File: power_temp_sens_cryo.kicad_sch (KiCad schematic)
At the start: 20 parts, among them J1 temp. sens., J2 MCU_ADC1, J3 MCU_ADC0, J4 5V, J5 GND, U1 AD8276, U2 AD8603, U3 AD8276, U4 AD8603

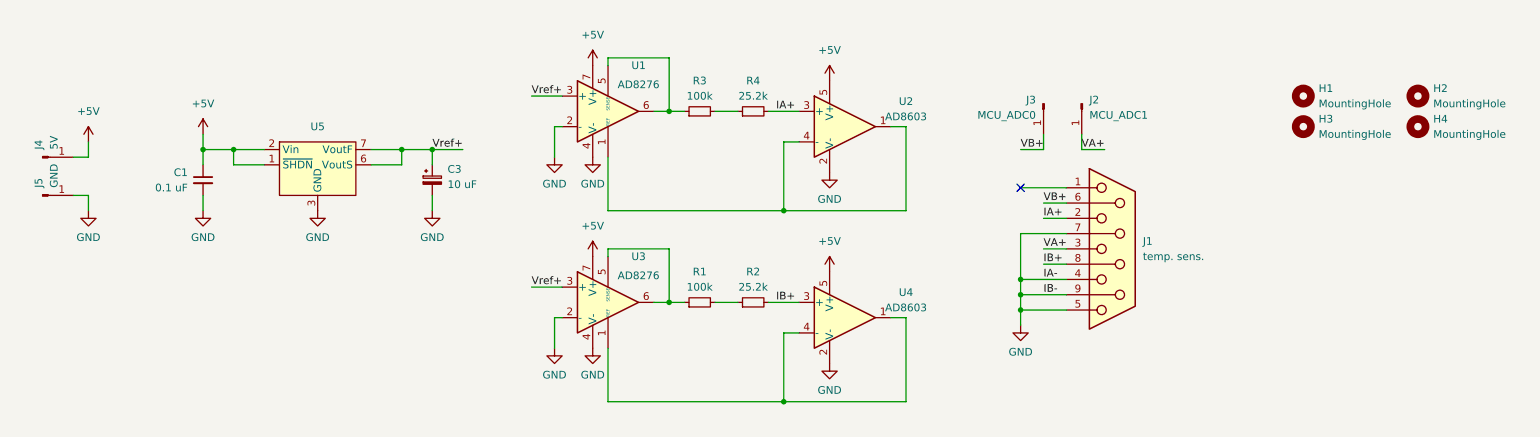
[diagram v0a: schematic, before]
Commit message: unfinished project
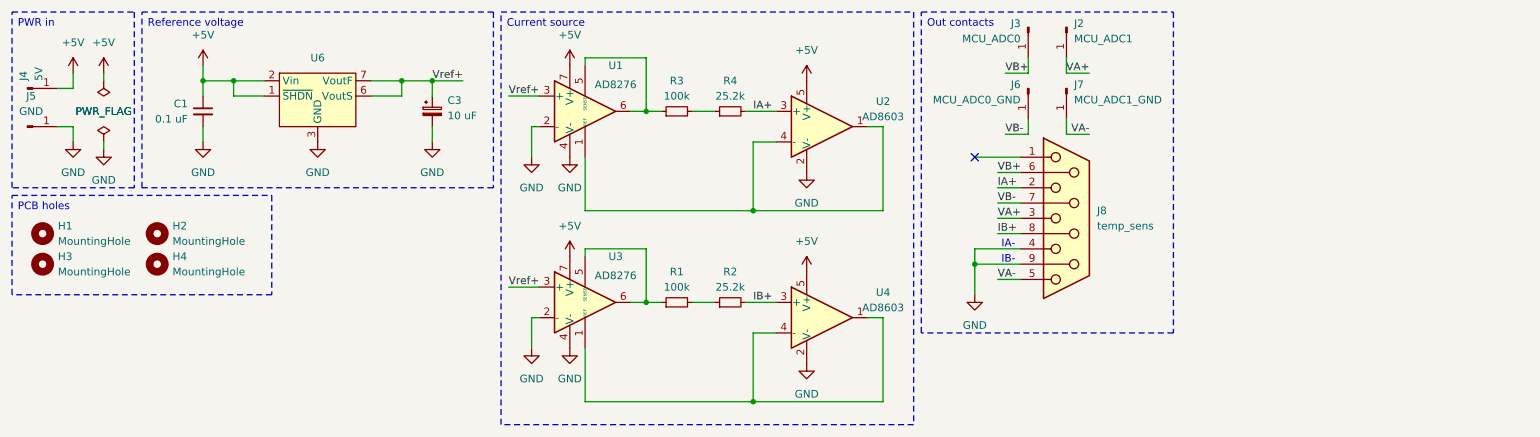
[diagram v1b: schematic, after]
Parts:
- removed J1: temp. sens., symbol Connector_self:DB9_Female
- removed U5: ~, Capacitor_SMD:CP_Elec_4x5.4, symbol ref:LTC6655
- added J6: MCU_ADC0_GND, Connector_PinHeader_2.54mm:PinHeader_1x01_P2.54mm_Vertical, symbol Connector:Conn_01x01_Pin
- added J7: MCU_ADC1_GND, Connector_PinHeader_2.54mm:PinHeader_1x01_P2.54mm_Vertical, symbol Connector:Conn_01x01_Pin
- added J8: temp_sens, symbol Connector:DE9_Socket
- added U6: ~, symbol ref:LTC6655
- J2, J3, J4, J5: footprint (none) -> Connector_PinHeader_2.54mm:PinHeader_1x01_P2.54mm_Vertical
- U1, U3: footprint (none) -> Package_SO:MSOP-8_3x3mm_P0.65mm
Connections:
- net +5V: now also U6.1 (~{SHDN}), U6.2 (Vin)
- net GND: now also J8.4, J8.9, U6.3 (GND), U6.4 (GND), U6.5 (GND), U6.8 (GND)
- net IA+: now also J8.2
- net IB+: now also J8.8
- net VA+: now also J8.3
- net VB+: now also J8.6
- net Vref+: now also U6.6 (VoutS), U6.7 (VoutF)
- new net VA-: J7.1 (Pin_1), J8.5
- new net VB-: J6.1 (Pin_1), J8.7
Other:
- note added: "IA-"
- note added: "IB-"
- moved on the sheet: C1, C3, H1, H2, H3, H4, J2, J3, J4, J5, R1, R2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
